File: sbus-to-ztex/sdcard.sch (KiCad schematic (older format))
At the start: 3 parts, among them J2 47219-2001

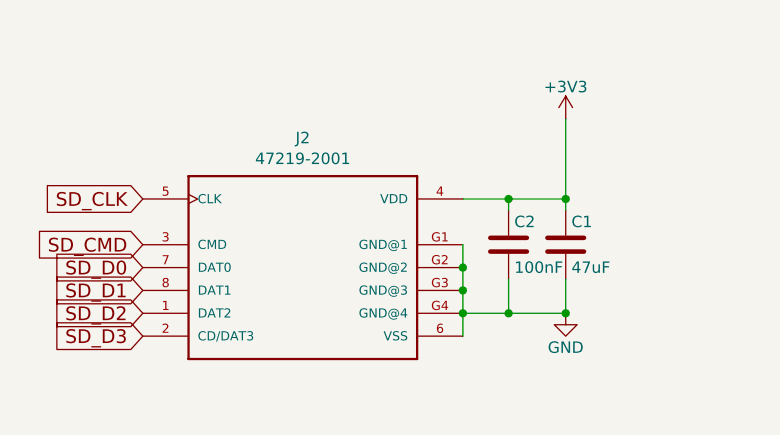
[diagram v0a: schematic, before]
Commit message: thinking about a V1.3
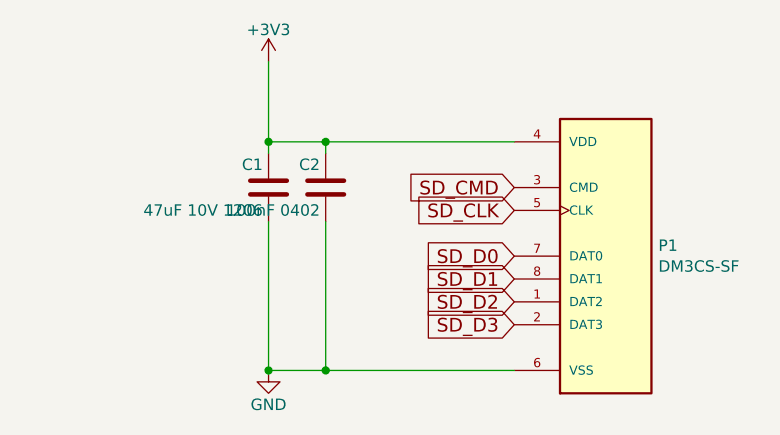
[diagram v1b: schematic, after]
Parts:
- removed J2: 47219-2001, MOLEX_47219-2001:MOLEX_47219-2001, symbol 47219-2001:47219-2001
- added P1: DM3CS-SF, For_SeeedStudio:HRS_DM3CS-SF, symbol DM3CS-SF:DM3CS-SF
- C1: value 47uF -> 47uF 10V 1206; footprint Capacitor_SMD:C_0805_2012Metric -> Capacitor_SMD:C_1206_3216Metric; MPN GRM21BR60J476ME15L -> CL31A476MPHNNNE; MPN-ALT (none) -> GRM21BR60J476ME15L; URL (none) -> https://www.lcsc.com/product-detail/Multilayer-Ceramic-Capa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; URL-ALT (none) -> https://www.lcsc.com/product-detail/Multilayer-Ceramic-Capa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
- C2: value 100nF -> 100nF 0402; footprint Capacitor_SMD:C_0603_1608Metric -> Capacitor_SMD:C_0402_1005Metric; LCSC ? -> (none); MNF1_URL www.yageo.com -> (none); MPN CC0603KRX7R8BB104 -> CL05B104KO5NNNC
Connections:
- net +3V3: now also P1.4 (VDD)
- net GND: now also P1.6 (VSS)
- net SD_CLK: now also P1.5 (CLK)
- net SD_CMD: now also P1.3 (CMD)
- net SD_D0: now also P1.7 (DAT0)
- net SD_D1: now also P1.8 (DAT1)
- net SD_D2: now also P1.1 (DAT2)
- net SD_D3: now also P1.2 (DAT3)
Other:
- moved on the sheet: C1, C2
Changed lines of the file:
@@
 EESchema Schematic File Version 4
-LIBS:sbus-to-ztex-cache
-EELAYER 26 0
+EELAYER 30 0
 EELAYER END
 $Descr A4 11693 8268
 encoding utf-8
-Sheet 5 6
+Sheet 5 9
 Title "sbus-to-ztex sdcard"
 Date ""
@@
 $EndDescr
 $Comp
-L power:GND #PWR0165
+L power:GND #PWR0103
 U 1 1 58DA7C71
-P 5450 5450
-F 0 "#PWR0165" H 5450 5200 50  0001 C CNN
-F 1 "GND" H 5450 5300 50  0000 C CNN
-F 2 "" H 5450 5450 50  0000 C CNN
-F 3 "" H 5450 5450 50  0000 C CNN
-	1    5450 5450
-	1    0    0    -1
+P 4150 5700
+F 0 "#PWR0103" H 4150 5450 50  0001 C CNN
+F 1 "GND" H 4150 5550 50  0000 C CNN
+F 2 "" H 4150 5700 50  0000 C CNN
+F 3 "" H 4150 5700 50  0000 C CNN
+	1    4150 5700
+	-1   0    0    -1
 $EndComp
 $Comp
-L power:+3V3 #PWR0166
+L power:+3V3 #PWR0135
 U 1 1 58DA7C72
-P 5450 4600
-F 0 "#PWR0166" H 5450 4450 50  0001 C CNN
-F 1 "+3V3" H 5450 4740 50  0000 C CNN
-F 2 "" H 5450 4600 50  0000 C CNN
-F 3 "" H 5450 4600 50  0000 C CNN
-	1    5450 4600
-	1    0    0    -1
+P 4150 4350
+F 0 "#PWR0135" H 4150 4200 50  0001 C CNN
+F 1 "+3V3" H 4150 4490 50  0000 C CNN
+F 2 "" H 4150 4350 50  0000 C CNN
+F 3 "" H 4150 4350 50  0000 C CNN
+	1    4150 4350
+	-1   0    0    -1
 $EndComp
-Text GLabel 3600 5450 0    60   Input ~ 0
+Text GLabel 5225 5400 0    60   Input ~ 0
 SD_D2
-Text GLabel 3600 5550 0    60   Input ~ 0
+Text GLabel 5225 5500 0    60   Input ~ 0
 SD_D3
-Text GLabel 3600 5150 0    60   Input ~ 0
+Text GLabel 5225 4900 0    60   Input ~ 0
 SD_CMD
-Text GLabel 3600 4950 0    60   Input ~ 0
+Text GLabel 5225 5000 0    60   Input ~ 0
 SD_CLK
-Text GLabel 3600 5250 0    60   Input ~ 0
+Text GLabel 5225 5200 0    60   Input ~ 0
 SD_D0
-Text GLabel 3600 5350 0    60   Input ~ 0
+Text GLabel 5225 5300 0    60   Input ~ 0
 SD_D1
 $Comp
 L Device:C C1
 U 1 1 590C7447
-P 5450 5150
-F 0 "C1" H 5475 5250 50  0000 L CNN
-F 1 "47uF" H 5475 5050 50  0000 L CNN
-F 2 "Capacitor_SMD:C_0805_2012Metric" H 5488 5000 50  0001 C CNN
-F 3 "" H 5450 5150 50  0000 C CNN
-F 4 "GRM21BR60J476ME15L" H 5450 5150 50  0001 C CNN "MPN"
-	1    5450 5150
-	1    0    0    -1
+P 4150 4900
+F 0 "C1" H 4175 5000 50  0000 L CNN
+F 1 "47uF 10V 1206" H 4175 4800 50  0000 L CNN
+F 2 "Capacitor_SMD:C_1206_3216Metric" H 4188 4750 50  0001 C CNN
+F 3 "" H 4150 4900 50  0000 C CNN
+F 4 "GRM21BR60J476ME15L" H 4150 4900 50  0001 C CNN "MPN-ALT"
+F 5 "https://www.lcsc.com/product-detail/Multilayer-Ceramic-Capacitors-MLCC-SMD-SMT_Murata-Electronics-GRM21BR60J476ME15L_C77072.html" H 4150 4900 50  0001 C CNN "URL-ALT"
+F 6 "CL31A476MPHNNNE" H 4150 4900 50  0001 C CNN "MPN"
+F 7 "https://www.lcsc.com/product-detail/Multilayer-Ceramic-Capacitors-MLCC-SMD-SMT_Samsung-Electro-Mechanics-CL31A476MPHNNNE_C96123.html" H 4150 4900 50  0001 C CNN "URL"
+	1    4150 4900
+	-1   0    0    -1
 $EndComp
+Wire Wire Line
+	4150 5700 4400 5700
+Connection ~ 4150 5700
+Connection ~ 4150 4700
+Wire Wire Line
+	4150 4700 4150 4750
 $Comp
-L 47219-2001:47219-2001 J2
-U 1 1 5F6F557B
-P 4300 5250
-F 0 "J2" H 4300 5817 50  0000 C CNN
-F 1 "47219-2001" H 4300 5726 50  0000 C CNN
-F 2 "MOLEX_47219-2001:MOLEX_47219-2001" H 4300 5250 50  0001 L BNN
-F 3 "https://www.molex.com/webdocs/datasheets/pdf/en-us/0472192001_MEMORY_CARD_SOCKET.pdf" H 4300 5250 50  0001 L BNN
-F 4 "47219-2001" H 4300 5250 50  0001 C CNN "MPN"
-	1    4300 5250
+L Device:C C?
+U 1 1 60D77AD6
+P 4400 4900
+AR Path="/5F679B53/60D77AD6" Ref="C?"  Part="1"
+AR Path="/5F69F4EF/60D77AD6" Ref="C2"  Part="1"
+AR Path="/619D66B7/60D77AD6" Ref="C15"  Part="1"
+AR Path="/62D70B59/60D77AD6" Ref="C9"  Part="1"
+F 0 "C2" H 4425 5000 50  0000 L CNN
+F 1 "100nF 0402" H 4425 4800 50  0000 L CNN
+F 2 "Capacitor_SMD:C_0402_1005Metric" H 4438 4750 50  0001 C CNN
+F 3 "" H 4400 4900 50  0000 C CNN
+F 4 "" H 4400 4900 50  0001 C CNN "MNF1_URL"
+F 5 "CL05B104KO5NNNC" H 4400 4900 50  0001 C CNN "MPN"
+F 6 "603-CC603KRX7R8BB104" H 4400 4900 50  0001 C CNN "Mouser"
+F 7 "?" H 4400 4900 50  0001 C CNN "Digikey"
+F 8 "" H 4400 4900 50  0001 C CNN "LCSC"
+F 9 "?" H 4400 4900 50  0001 C CNN "Koncar"
+F 10 "TB" H 4400 4900 50  0001 C CNN "Side"
+F 11 "" H 2200 5800 50  0001 C CNN "URL"
+	1    4400 4900
+	-1   0    0    -1
+$EndComp
+Wire Wire Line
+	4400 4750 4400 4700
+Connection ~ 4400 4700
+Wire Wire Line
+	4400 4700 4150 4700
+Connection ~ 4400 5700
+Wire Wire Line
+	4150 4350 4150 4700
+$Comp
+L DM3CS-SF:DM3CS-SF P1
+U 1 1 641CE916
+P 5525 5200
+F 0 "P1" H 5855 5246 50  0000 L CNN
+F 1 "DM3CS-SF" H 5855 5155 50  0000 L CNN
+F 2 "For_SeeedStudio:HRS_DM3CS-SF" H 5525 5200 50  0001 L BNN
+F 3 "" H 5525 5200 50  0001 L BNN
+F 4 "Hirose Electric Co Ltd" H 5525 5200 50  0001 L BNN "MANUFACTURER"
+F 5 "DM3CS-SF" H 5525 5200 50  0001 C CNN "MPN"
+F 6 "https://www.lcsc.com/product-detail/SD-Card-Connectors_HRS-Hirose-DM3CS-SF_C202111.html" H 5525 5200 50  0001 C CNN "URL"
+	1    5525 5200
 	1    0    0    -1
 $EndComp
 Wire Wire Line
-	5450 5450 5200 5450
+	4150 5050 4150 5700
 Wire Wire Line
-	5000 5450 5000 5350
-Connection ~ 5000 5450
+	4400 5050 4400 5700
 Wire Wire Line
-	5000 5350 5000 5250
-Connection ~ 5000 5350
+	4400 5700 5225 5700
 Wire Wire Line
-	5000 5250 5000 5150
-Connection ~ 5000 5250
-Wire Wire Line
-	5000 5550 5000 5450
-Wire Wire Line
-	5450 5300 5450 5450
-Connection ~ 5450 5450
-Wire Wire Line
-	5000 4950 5200 4950
-Connection ~ 5450 4950
-Wire Wire Line
-	5450 4950 5450 5000
-$Comp
-L Device:C C?
-U 1 1 60D77AD6
-P 5200 5150
-AR Path="/5F679B53/60D77AD6" Ref="C?"  Part="1"
-AR Path="/5F69F4EF/60D77AD6" Ref="C2"  Part="1"
-F 0 "C2" H 5225 5250 50  0000 L CNN
-F 1 "100nF" H 5225 5050 50  0000 L CNN
-F 2 "Capacitor_SMD:C_0603_1608Metric" H 5238 5000 50  0001 C CNN
-F 3 "" H 5200 5150 50  0000 C CNN
-F 4 "www.yageo.com" H 5200 5150 50  0001 C CNN "MNF1_URL"
-F 5 "CC0603KRX7R8BB104" H 5200 5150 50  0001 C CNN "MPN"
-F 6 "603-CC603KRX7R8BB104" H 5200 5150 50  0001 C CNN "Mouser"
-F 7 "?" H 5200 5150 50  0001 C CNN "Digikey"
-F 8 "?" H 5200 5150 50  0001 C CNN "LCSC"
-F 9 "?" H 5200 5150 50  0001 C CNN "Koncar"
-F 10 "TB" H 5200 5150 50  0001 C CNN "Side"
-	1    5200 5150
-	1    0    0    -1
-$EndComp
-Wire Wire Line
-	5200 5000 5200 4950
-Connection ~ 5200 4950
-Wire Wire Line
-	5200 4950 5450 4950
-Wire Wire Line
-	5200 5300 5200 5450
-Connection ~ 5200 5450
-Wire Wire Line
-	5200 5450 5000 5450
-Wire Wire Line
-	5450 4600 5450 4950
+	4400 4700 5225 4700
 $EndSCHEMATC
